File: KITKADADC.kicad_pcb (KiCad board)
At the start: 2 copper layers, 87 parts, among them U35 MCP6004, U36 MCP6004, U46 MCP6004, U8 MCP6004

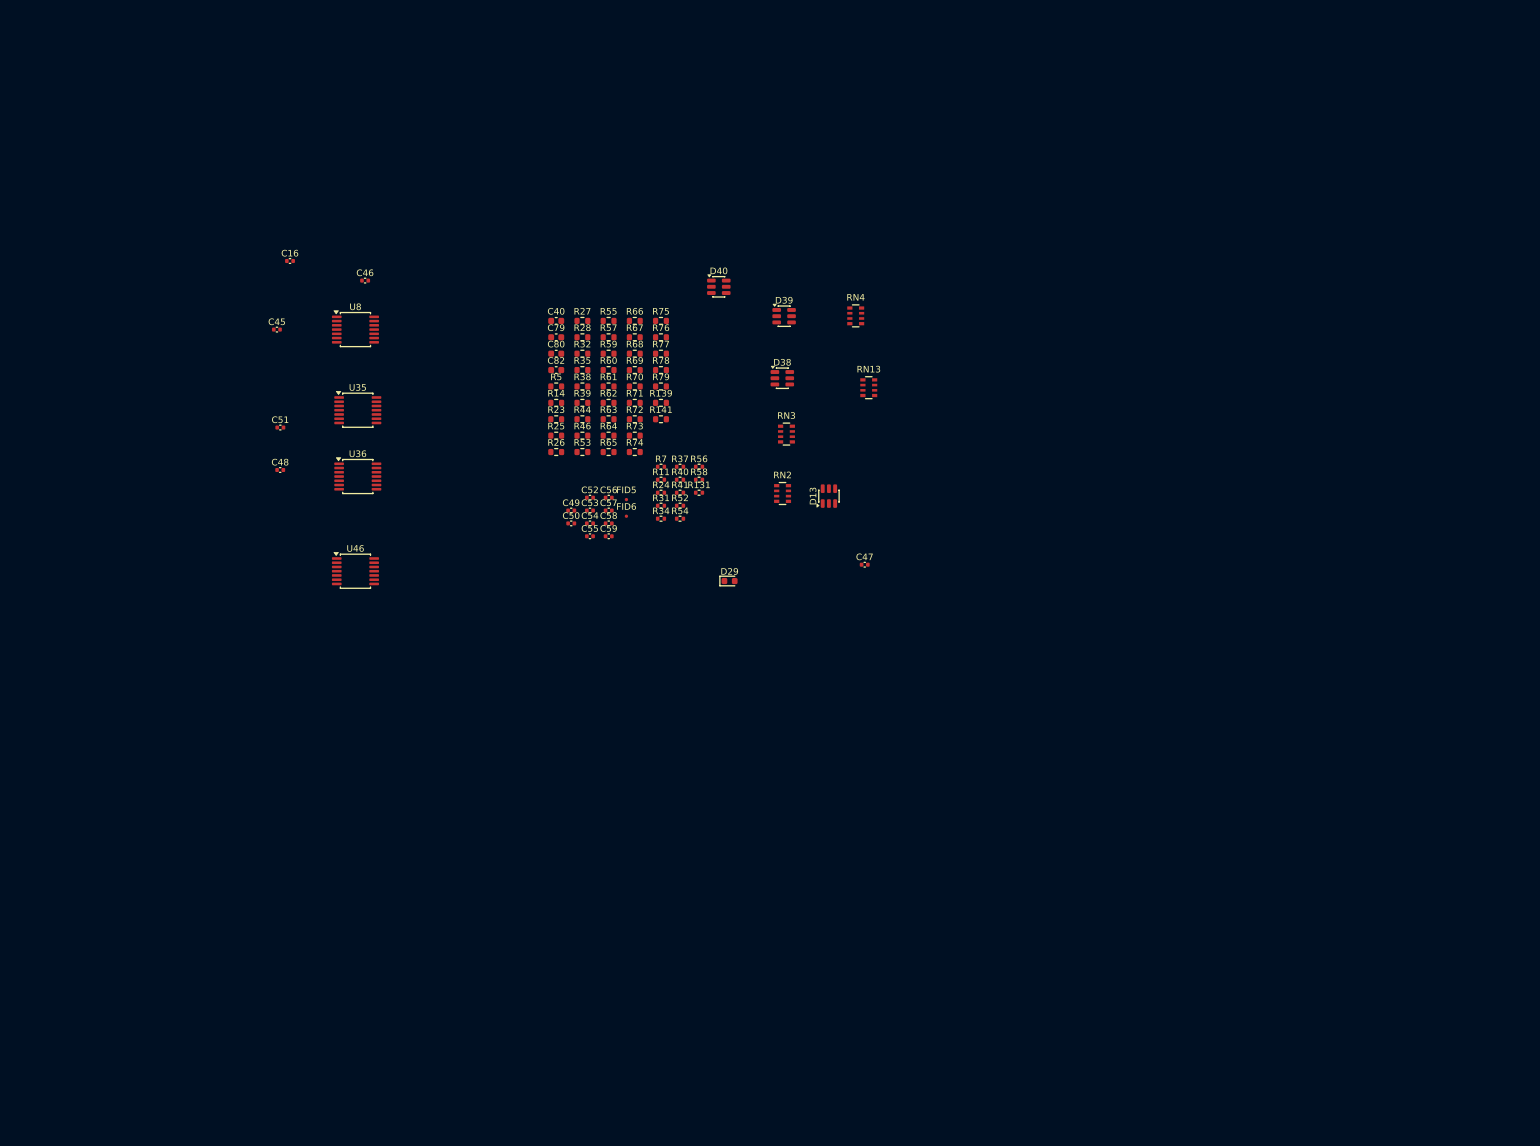
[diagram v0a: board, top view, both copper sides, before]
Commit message: ordenando
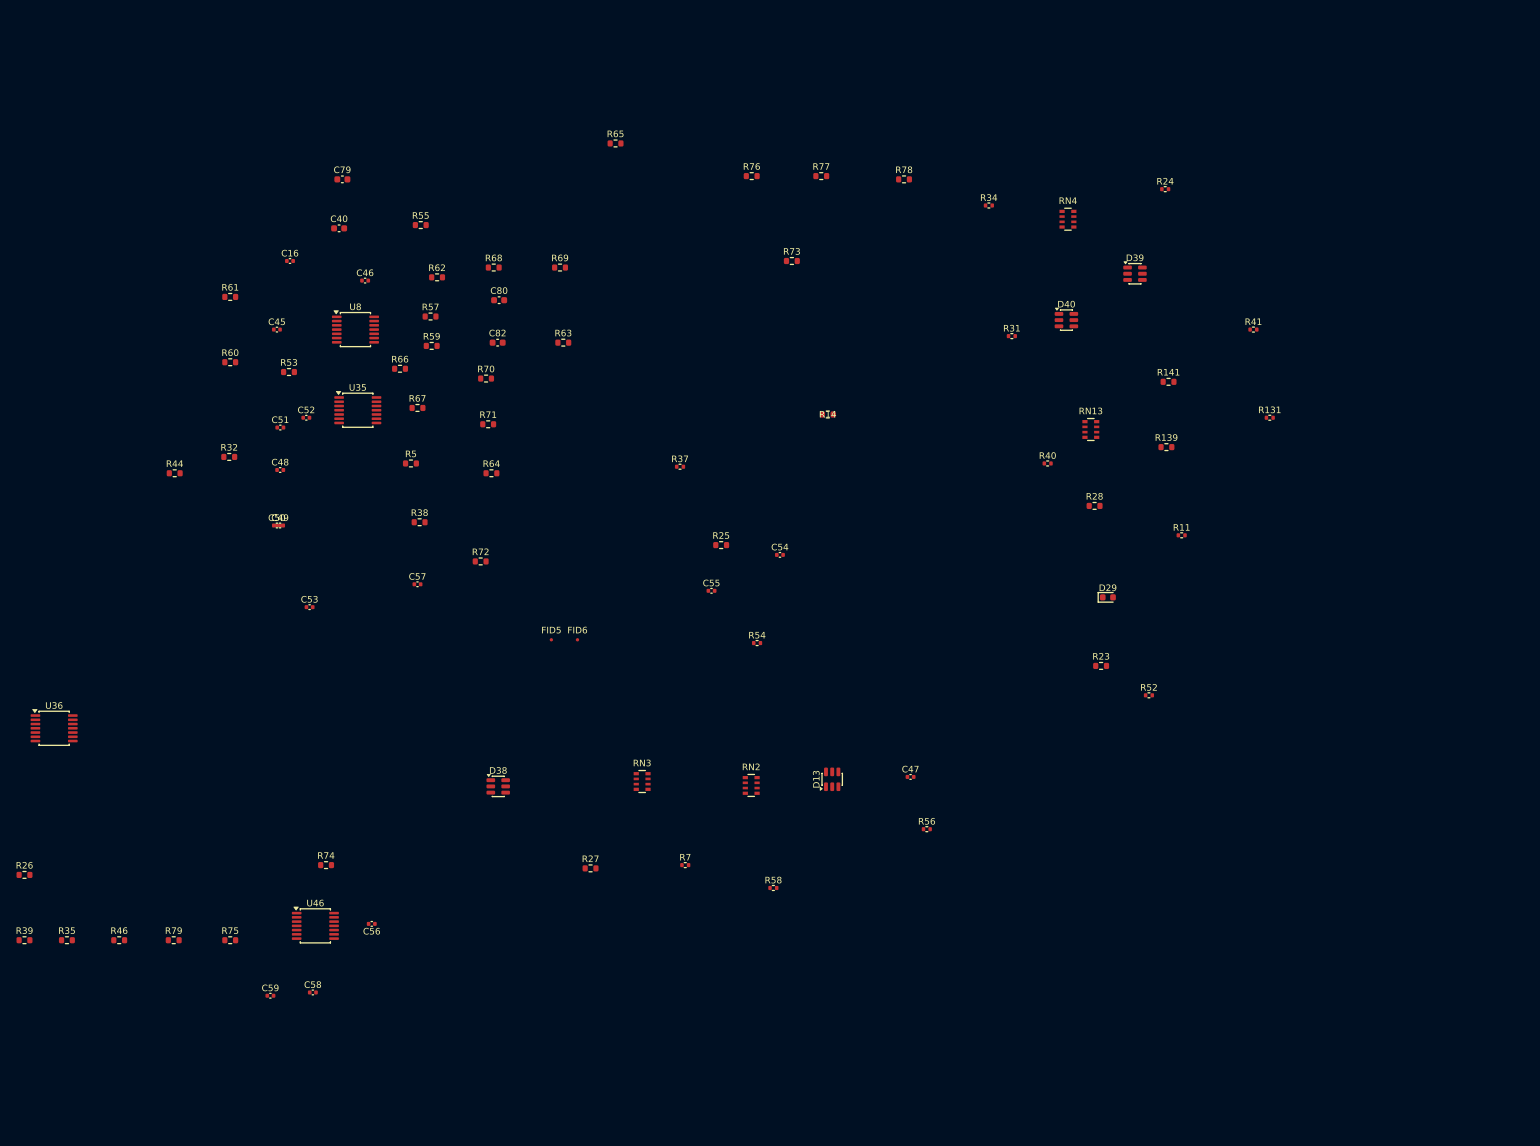
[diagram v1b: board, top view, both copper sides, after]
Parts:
- moved R39 118.6 mm to (24.3, 163.5)
- moved R35 117.7 mm to (30.8, 163.5)
- moved R75 115.5 mm to (55.8, 163.5)
- moved R79 112.9 mm to (47.2, 163.5)
- moved R46 104.9 mm to (38.8, 163.5)
- moved R26 104.0 mm to (24.3, 153.5)
- moved R23 91.6 mm to (189.2, 121.5)
- moved R41 91.3 mm to (212.5, 70.0)
- moved R24 90.1 mm to (199.0, 48.5)
- moved R131 88.1 mm to (215.0, 83.5)
- moved C59 87.4 mm to (62.0, 172.0)
- moved C58 84.9 mm to (68.5, 171.5)
- moved R27 83.8 mm to (111.0, 152.5)
- moved R28 82.6 mm to (188.2, 97.0)
- moved R11 80.2 mm to (201.5, 101.5)
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
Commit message: recolocando pcb
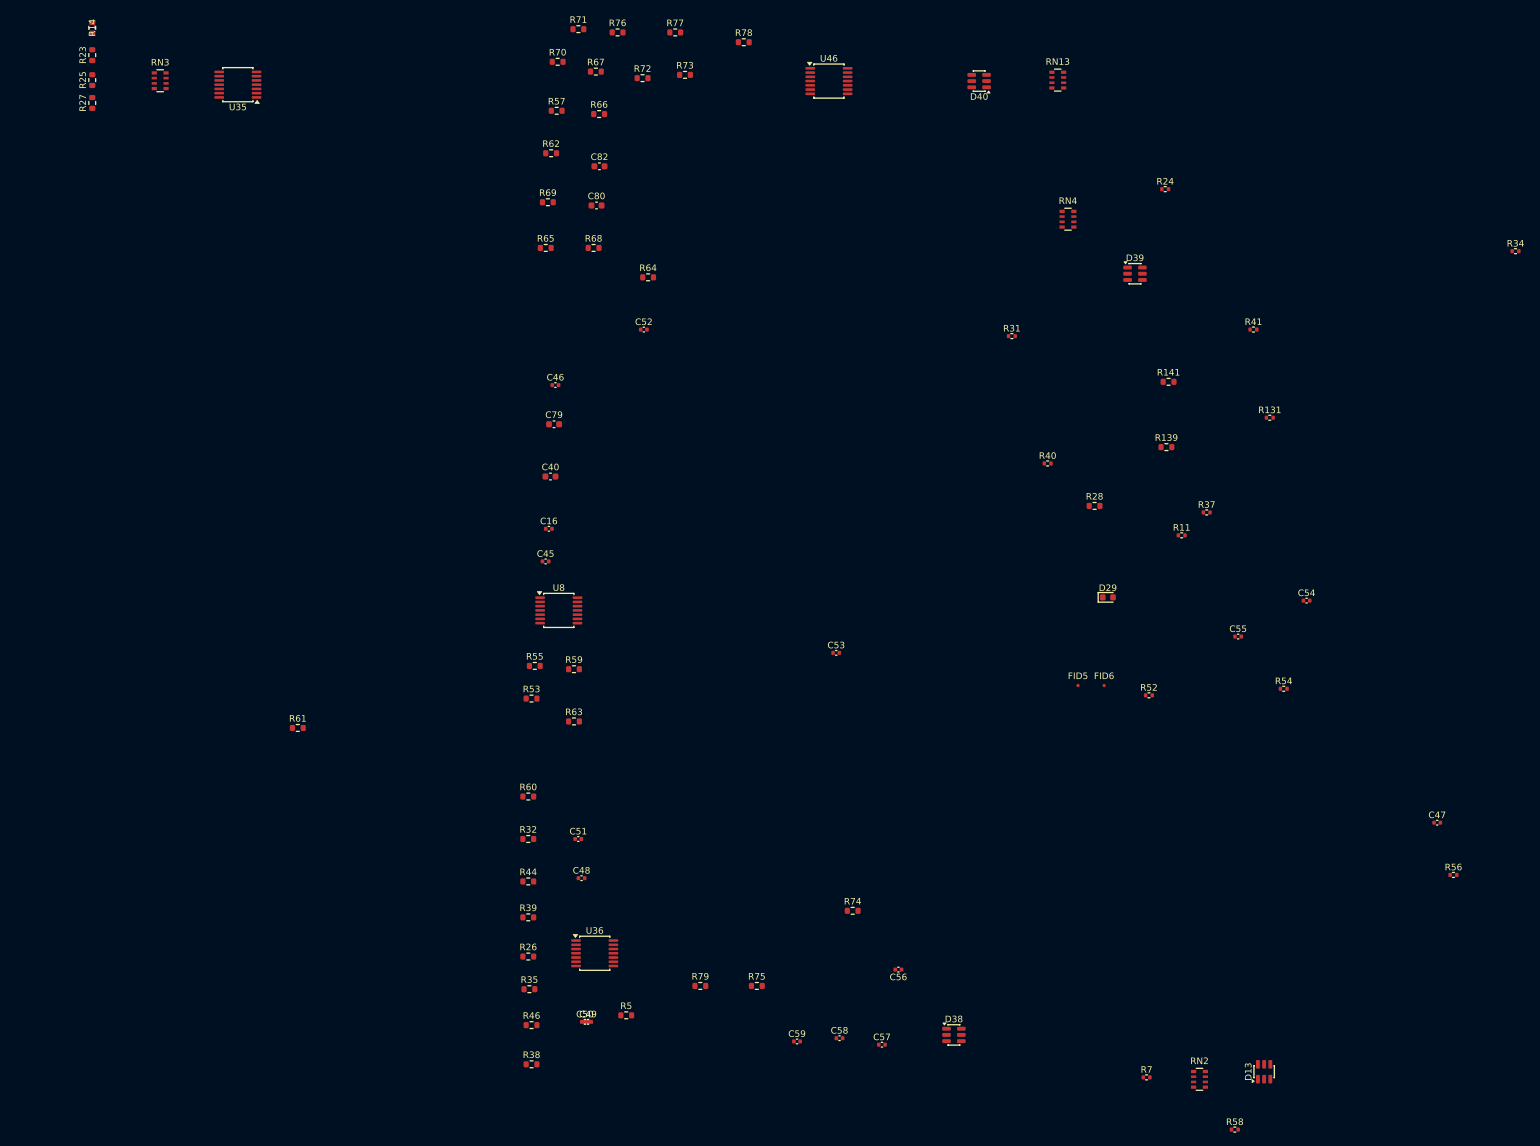
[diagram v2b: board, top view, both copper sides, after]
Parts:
- moved R23 180.6 mm to (34.7, 28.0), turned to 90 degrees
- moved U46 151.4 mm to (147.5, 31.9)
- moved R27 139.8 mm to (34.7, 35.3), turned to 90 degrees
- moved RN3 130.2 mm to (45.1, 31.9)
- moved R14 127.2 mm to (34.7, 23.8), turned to -90 degrees
- moved R25 119.8 mm to (34.7, 31.8), turned to 90 degrees
- moved C57 100.1 mm to (155.6, 179.5)
- moved R5 90.7 mm to (116.5, 175.0)
- moved U36 89.7 mm to (111.6, 165.5)
- moved C49 89.4 mm to (110.6, 176.0)
- moved C50 89.4 mm to (110.1, 176.0)
- moved R38 84.8 mm to (102.0, 182.5)
- moved R44 82.7 mm to (101.5, 154.5)
- moved RN2 82.1 mm to (204.2, 184.8)
- moved C59 80.9 mm to (142.6, 179.0)
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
